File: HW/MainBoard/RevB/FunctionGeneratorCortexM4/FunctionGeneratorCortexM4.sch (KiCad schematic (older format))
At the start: 2 parts, among them J1 Conn_02x05_Odd_Even, J2 Screw_Terminal_01x02

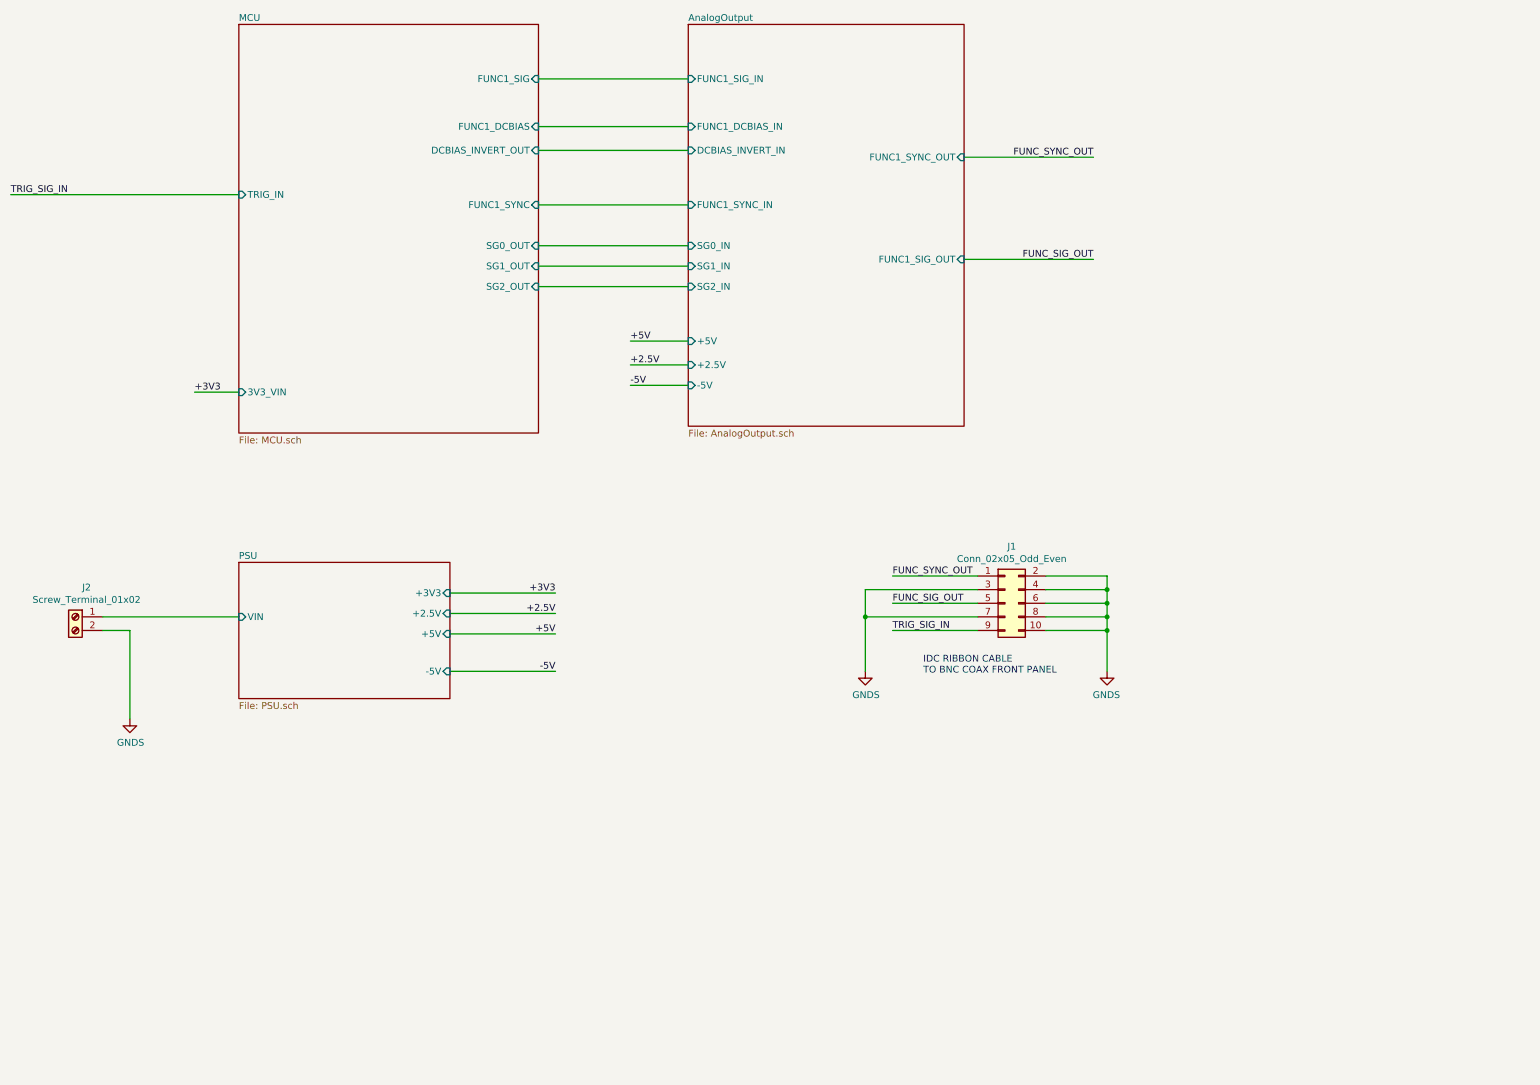
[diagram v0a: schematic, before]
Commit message: OPTIMIZED REVB LAYOUT
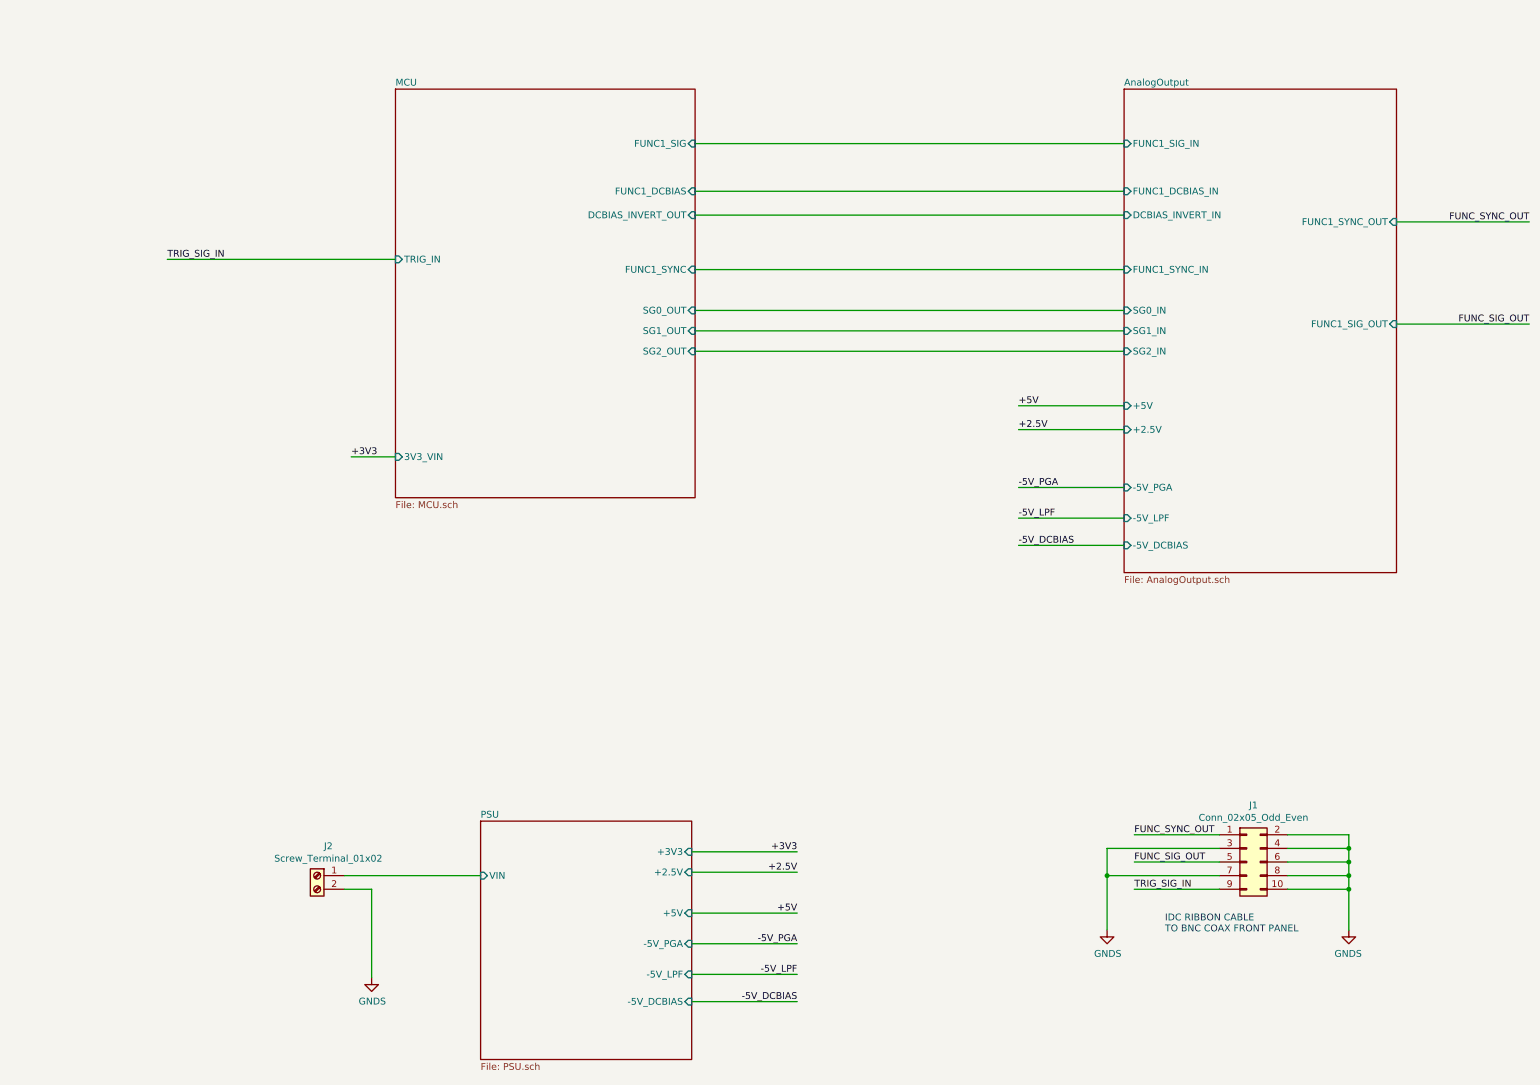
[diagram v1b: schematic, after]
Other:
- moved on the sheet: J1, J2
